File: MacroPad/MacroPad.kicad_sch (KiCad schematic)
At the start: 27 parts, among them SW1 CherryMX, SW10 CherryMX, SW11 CherryMX, SW12 CherryMX, SW2 CherryMX, SW3 CherryMX, SW4 CherryMX, SW5 CherryMX, SW6 CherryMX, SW7 CherryMX, SW8 CherryMX, SW9 CherryMX, U1 ESP32-DevKitC

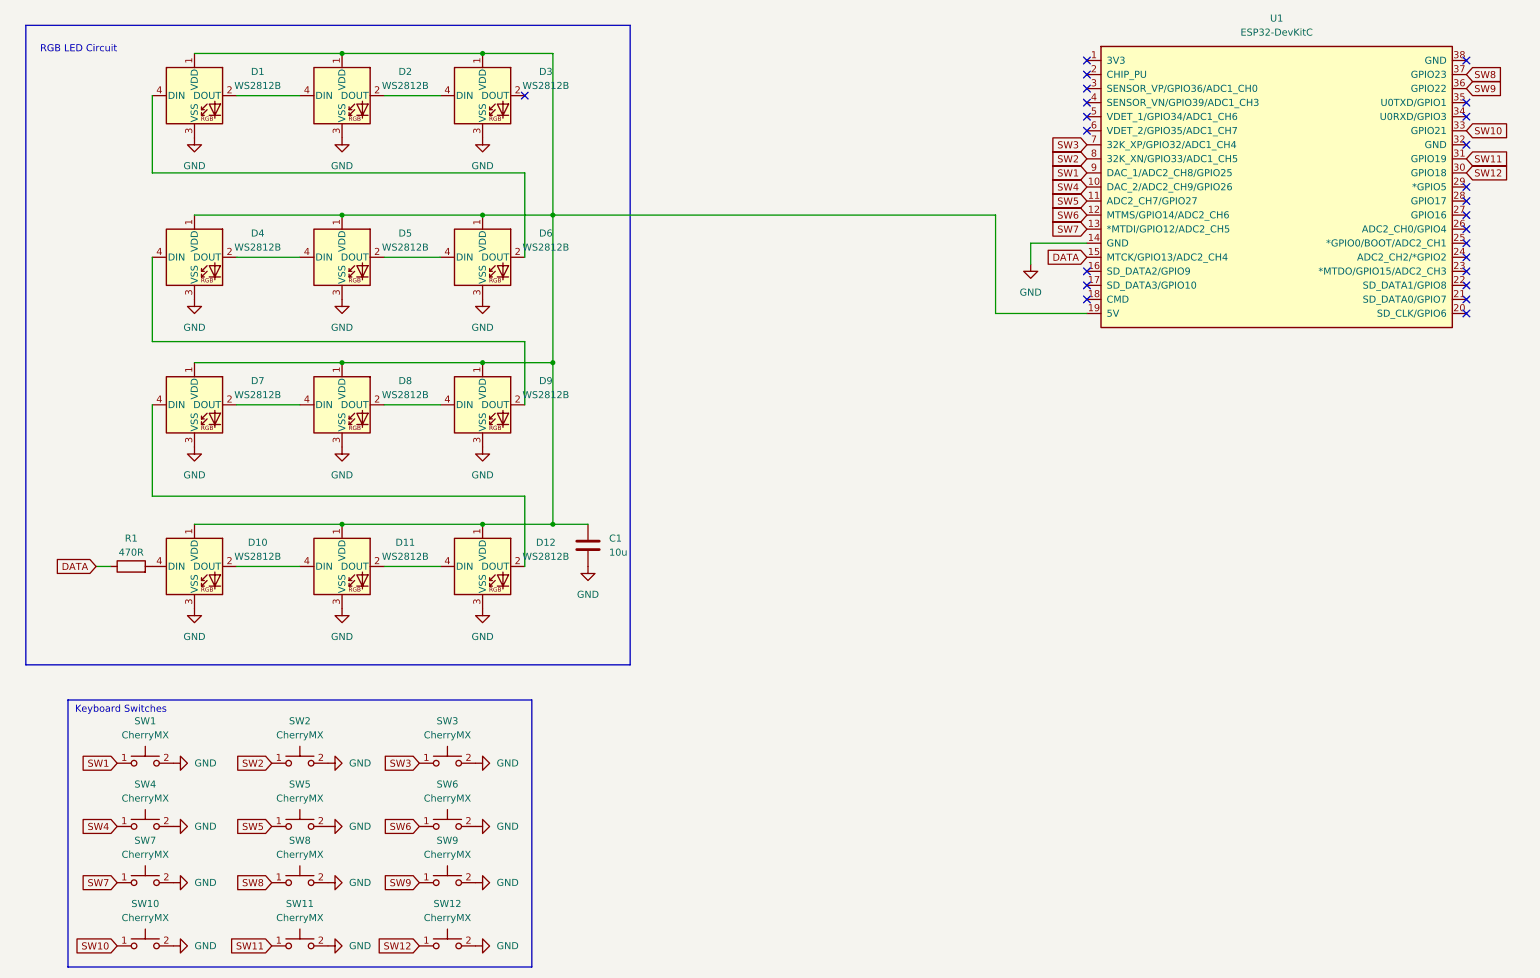
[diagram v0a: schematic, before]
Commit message: Finished PCB i think
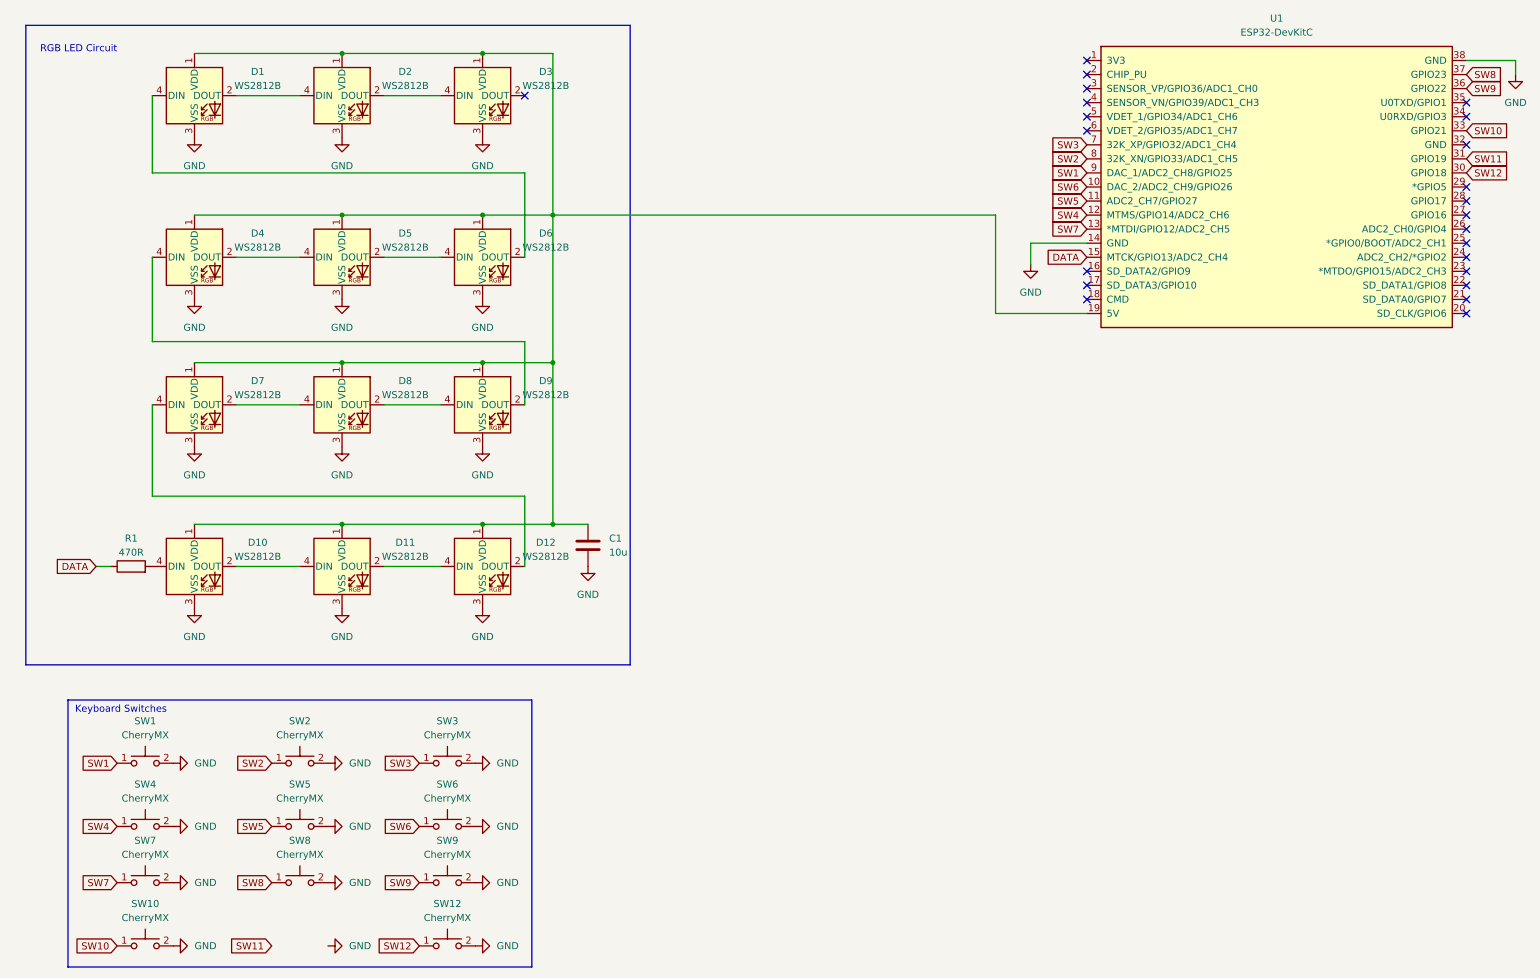
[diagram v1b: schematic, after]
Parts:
- removed SW11: CherryMX, Switch_Keyboard_Cherry_MX:SW_Cherry_MX_Plate_1.00u, symbol CherryMX:CherryMX
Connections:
- net GND: now also U1.38 (GND)
- net SW4: now also U1.12 (MTMS/GPIO14/ADC2_CH6); no longer U1.10 (DAC_2/ADC2_CH9/GPIO26)
- net SW6: now also U1.10 (DAC_2/ADC2_CH9/GPIO26); no longer U1.12 (MTMS/GPIO14/ADC2_CH6)
- no-connect marks 24 -> 23
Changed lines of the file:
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@@
   (no_connect (at 274.32 62.23))
   (no_connect (at 274.32 57.15))
-  (no_connect (at 274.32 26.67))
   (no_connect (at 104.14 33.02))
   (no_connect (at 205.74 64.77))
@@
     (stroke (width 0) (type default) (color 0 0 0 0))
   )
+  (wire (pts (xy 274.32 26.67) (xy 283.21 26.67))
+    (stroke (width 0) (type default) (color 0 0 0 0))
+  )
   (polyline (pts (xy 123.19 20.32) (xy 123.19 135.89))
     (stroke (width 0) (type default) (color 0 0 0 0))
@@
   )
   (wire (pts (xy 96.52 81.28) (xy 109.22 81.28))
+    (stroke (width 0) (type default) (color 0 0 0 0))
+  )
+  (wire (pts (xy 283.21 26.67) (xy 283.21 29.21))
     (stroke (width 0) (type default) (color 0 0 0 0))
   )
@@
     )
   )
-  (global_label "SW6" (shape input) (at 205.74 54.61 180) (fields_autoplaced)
-    (effects (font (size 1.27 1.27)) (justify right))
-    (property "Intersheet References" "${INTERSHEET_REFS}" (id 0) (at 199.4564 54.5306 0)
+  (global_label "SW6" (shape input) (at 205.74 49.53 180) (fields_autoplaced)
+    (effects (font (size 1.27 1.27)) (justify right))
+    (property "Intersheet References" "${INTERSHEET_REFS}" (id 0) (at 199.4564 49.4506 0)
       (effects (font (size 1.27 1.27)) (justify right) hide)
     )
@@
     )
   )
-  (global_label "SW4" (shape input) (at 205.74 49.53 180) (fields_autoplaced)
-    (effects (font (size 1.27 1.27)) (justify right))
-    (property "Intersheet References" "${INTERSHEET_REFS}" (id 0) (at 199.4564 49.4506 0)
+  (global_label "SW4" (shape input) (at 205.74 54.61 180) (fields_autoplaced)
+    (effects (font (size 1.27 1.27)) (justify right))
+    (property "Intersheet References" "${INTERSHEET_REFS}" (id 0) (at 199.4564 54.5306 0)
       (effects (font (size 1.27 1.27)) (justify right) hide)
     )
@@
     )
     (property "Datasheet" "" (id 3) (at 44.45 40.64 0)
+      (effects (font (size 1.27 1.27)) hide)
+    )
+    (pin "1")
+  )
+  (symbol (lib_id "power:GND") (at 283.21 29.21 0) (unit 1)
+    (in_bom yes) (on_board yes) (fields_autoplaced)
+    (property "Reference" "#PWR?" (id 0) (at 283.21 35.56 0)
+      (effects (font (size 1.27 1.27)) hide)
+    )
+    (property "Value" "GND" (id 1) (at 283.21 34.29 0))
+    (property "Footprint" "" (id 2) (at 283.21 29.21 0)
+      (effects (font (size 1.27 1.27)) hide)
+    )
+    (property "Datasheet" "" (id 3) (at 283.21 29.21 0)
       (effects (font (size 1.27 1.27)) hide)
     )
@@
     (pin "1")
   )
-  (symbol (lib_id "CherryMX:CherryMX") (at 63.5 186.69 0) (unit 1)
-    (in_bom yes) (on_board yes) (fields_autoplaced)
-    (property "Reference" "SW11" (id 0) (at 63.5 179.07 0))
-    (property "Value" "CherryMX" (id 1) (at 63.5 181.61 0))
-    (property "Footprint" "Switch_Keyboard_Cherry_MX:SW_Cherry_MX_Plate_1.00u" (id 2) (at 63.5 186.055 0)
-      (effects (font (size 1.27 1.27)) hide)
-    )
-    (property "Datasheet" "" (id 3) (at 63.5 186.055 0)
-      (effects (font (size 1.27 1.27)) hide)
-    )
-    (pin "1")
-    (pin "2")
-  )
   (symbol (lib_id "CherryMX:CherryMX") (at 35.56 165.1 0) (unit 1)
     (in_bom yes) (on_board yes) (fields_autoplaced)
@@
       (reference "#PWR0126") (unit 1) (value "GND") (footprint "")
     )
+    (path "/34e41f35-7545-4f1a-8fb0-63e57b3abf99"
+      (reference "#PWR?") (unit 1) (value "GND") (footprint "")
+    )
     (path "/f46ec625-5522-41cc-be5f-679b6d2d5d61"
       (reference "C1") (unit 1) (value "10u") (footprint "Capacitor_SMD:C_1206_3216Metric_Pad1.33x1.80mm_HandSolder")
@@
       (reference "SW10") (unit 1) (value "CherryMX") (footprint "Switch_Keyboard_Cherry_MX:SW_Cherry_MX_Plate_1.00u")
     )
-    (path "/d0c21061-7bdc-4398-929e-fd92796a2721"
-      (reference "SW11") (unit 1) (value "CherryMX") (footprint "Switch_Keyboard_Cherry_MX:SW_Cherry_MX_Plate_1.00u")
-    )
     (path "/ca7e6571-12e2-46a7-8a55-d805e55d7c13"
